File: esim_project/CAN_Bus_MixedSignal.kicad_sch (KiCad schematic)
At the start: 12 parts, among them U1 adc_bridge_2, U2 adc_bridge_4, U3 can_node_top, U4 can_node_top, U5 dac_bridge_2, X1 can_phy

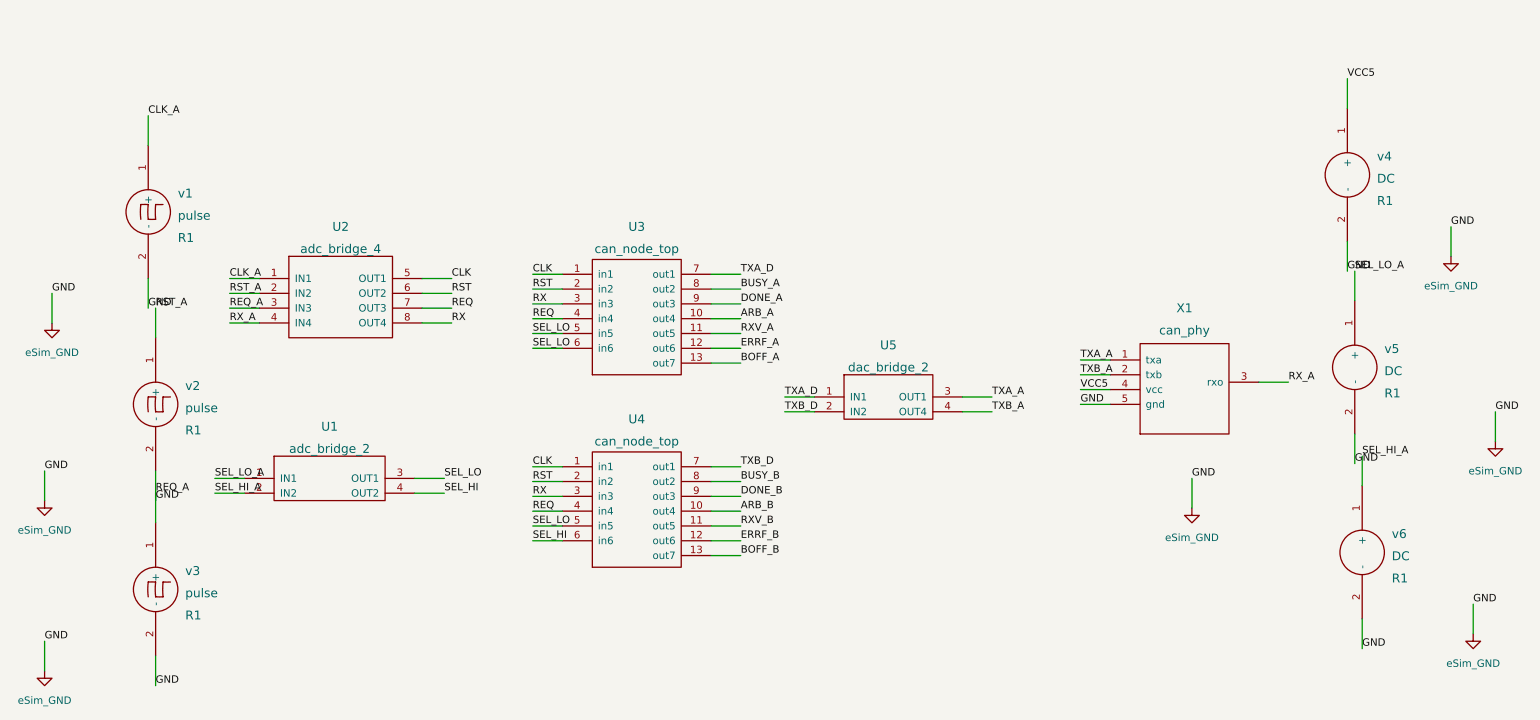
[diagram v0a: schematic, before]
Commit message: Day 42 final: schematic fully wired, netlist verified unchanged
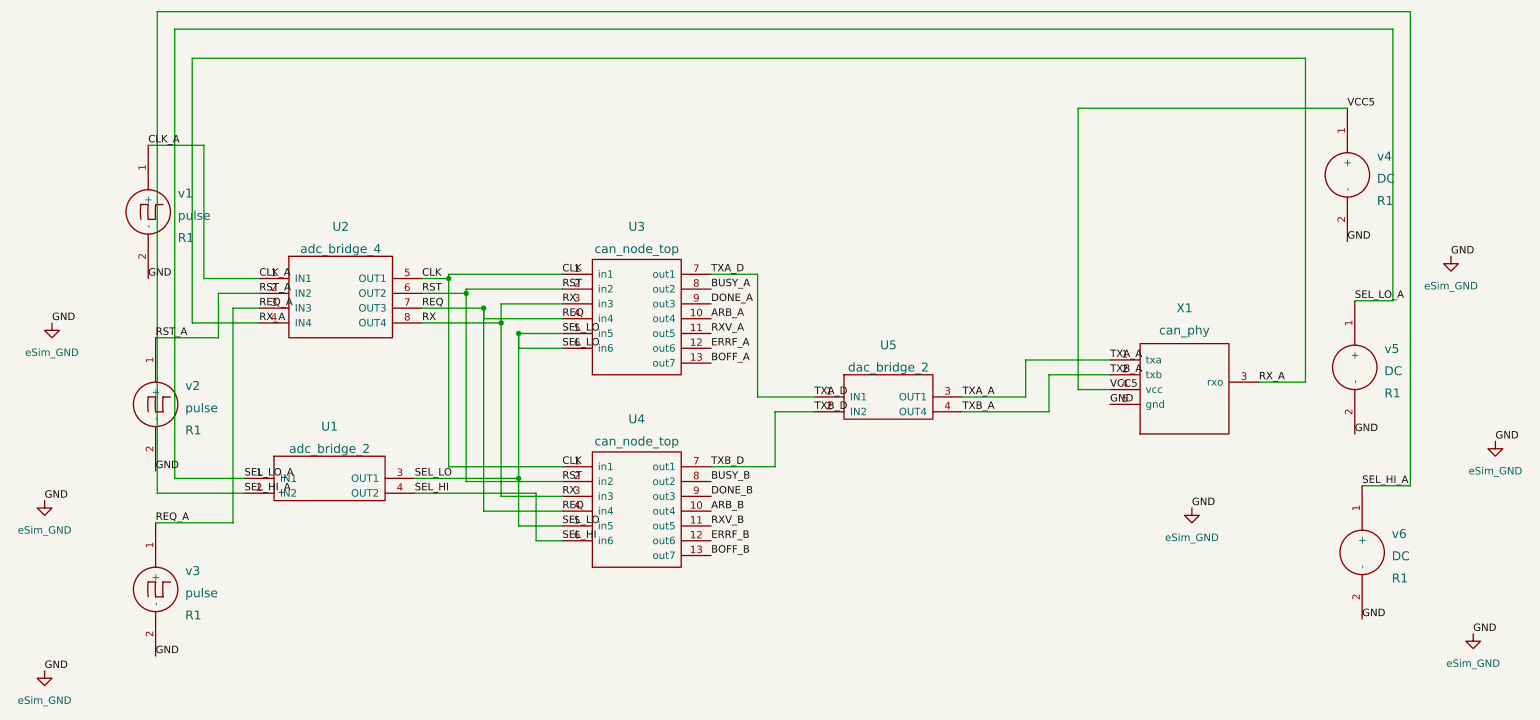
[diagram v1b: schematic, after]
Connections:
- net GND: no longer U2.3 (IN3), v3.1 (+)
- new net REQ_A: U2.3 (IN3), v3.1 (+)
